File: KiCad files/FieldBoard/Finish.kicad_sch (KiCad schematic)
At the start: 16 parts

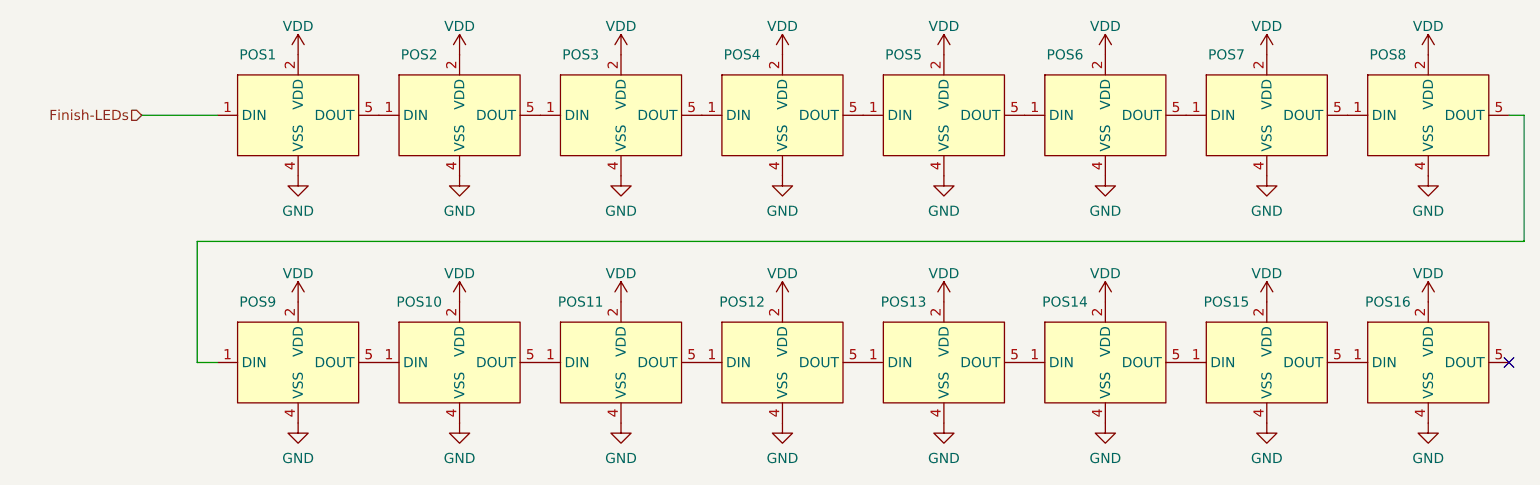
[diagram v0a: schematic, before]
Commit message: v2
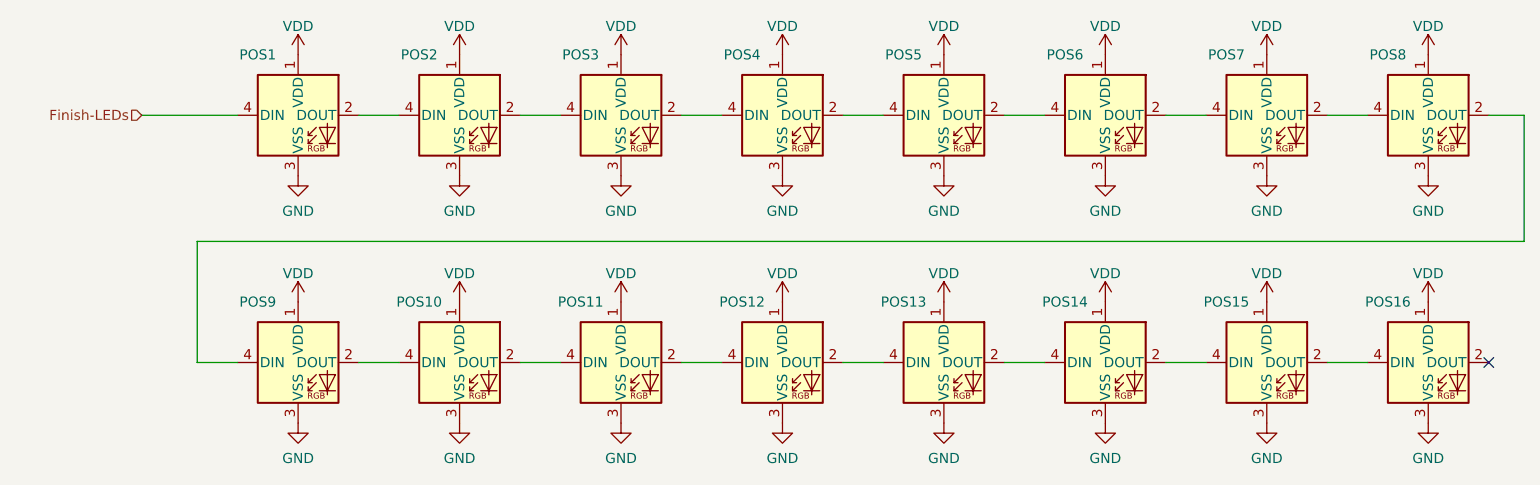
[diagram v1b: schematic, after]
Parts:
- POS1, POS10, POS11, POS12, POS13, POS14, POS16, POS2, POS3, POS4, POS5, POS6, POS7, POS8, POS9: footprint FieldBoard_footprint:WS2812-4020-dual-7mm_bezMaske -> LED_SMD:LED_WS2812B_PLCC4_5.0x5.0mm_P3.2mm; symbol FieldBoard_symbol:WS2812-4020_dual -> LED:WS2812B
- POS15: value WS2812-4020_dual -> (none); footprint FieldBoard_footprint:WS2812-4020-dual-7mm_bezMaske -> LED_SMD:LED_WS2812B_PLCC4_5.0x5.0mm_P3.2mm; symbol FieldBoard_symbol:WS2812-4020_dual -> LED:WS2812B
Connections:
- net Finish-LEDs: now also POS1.4 (DIN); no longer POS1.1 (DIN)
- net GND: now also POS1.3 (VSS), POS10.3 (VSS), POS11.3 (VSS), POS12.3 (VSS), POS13.3 (VSS), POS14.3 (VSS), POS15.3 (VSS), POS16.3 (VSS), POS2.3 (VSS), POS3.3 (VSS), POS4.3 (VSS), POS5.3 (VSS), POS6.3 (VSS), POS7.3 (VSS), POS8.3 (VSS), POS9.3 (VSS); no longer POS1.4 (VSS), POS10.4 (VSS), POS11.4 (VSS), POS12.4 (VSS), POS13.4 (VSS), POS14.4 (VSS), POS15.4 (VSS), POS16.4 (VSS), POS2.4 (VSS), POS3.4 (VSS), POS4.4 (VSS), POS5.4 (VSS), POS6.4 (VSS), POS7.4 (VSS), POS8.4 (VSS), POS9.4 (VSS)
- net VDD: now also POS1.1 (VDD), POS10.1 (VDD), POS11.1 (VDD), POS12.1 (VDD), POS13.1 (VDD), POS14.1 (VDD), POS15.1 (VDD), POS16.1 (VDD), POS2.1 (VDD), POS3.1 (VDD), POS4.1 (VDD), POS5.1 (VDD), POS6.1 (VDD), POS7.1 (VDD), POS8.1 (VDD), POS9.1 (VDD); no longer POS1.2 (VDD), POS10.2 (VDD), POS11.2 (VDD), POS12.2 (VDD), POS13.2 (VDD), POS14.2 (VDD), POS15.2 (VDD), POS16.2 (VDD), POS2.2 (VDD), POS3.2 (VDD), POS4.2 (VDD), POS5.2 (VDD), POS6.2 (VDD), POS7.2 (VDD), POS8.2 (VDD), POS9.2 (VDD)
- new net: POS13.2 (DOUT), POS14.4 (DIN)
- new net: POS12.2 (DOUT), POS13.4 (DIN)
- new net: POS7.2 (DOUT), POS8.4 (DIN)
- new net: POS6.2 (DOUT), POS7.4 (DIN)
- new net: POS2.2 (DOUT), POS3.4 (DIN)
- new net: POS1.2 (DOUT), POS2.4 (DIN)
- new net: POS8.2 (DOUT), POS9.4 (DIN)
- new net: POS10.2 (DOUT), POS11.4 (DIN)
- new net: POS10.4 (DIN), POS9.2 (DOUT)
- new net: POS15.2 (DOUT), POS16.4 (DIN)
- new net: POS14.2 (DOUT), POS15.4 (DIN)
- new net: POS11.2 (DOUT), POS12.4 (DIN)
- new net: POS5.2 (DOUT), POS6.4 (DIN)
- new net: POS4.2 (DOUT), POS5.4 (DIN)
- new net: POS3.2 (DOUT), POS4.4 (DIN)
